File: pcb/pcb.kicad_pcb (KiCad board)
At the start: 2 copper layers, 152 x 91.6 mm, 66 parts, among them J1 USB_C_Receptacle_USB2.0_16P, J2 Conn_01x02, K1 SW_Push, K10 SW_Push, K11 SW_Push, K12 SW_Push, K13 SW_Push, K14 SW_Push, K15 SW_Push, K16 SW_Push, K17 SW_Push, K18 SW_Push, K19 SW_Push, K2 SW_Push, K20 SW_Push, K21 SW_Push, K3 SW_Push, K4 SW_Push, K5 SW_Push, K6 SW_Push, K7 SW_Push, K8 SW_Push, K9 SW_Push, U1 SRV05-4, U2 ProMicro, U3 SRV05-4

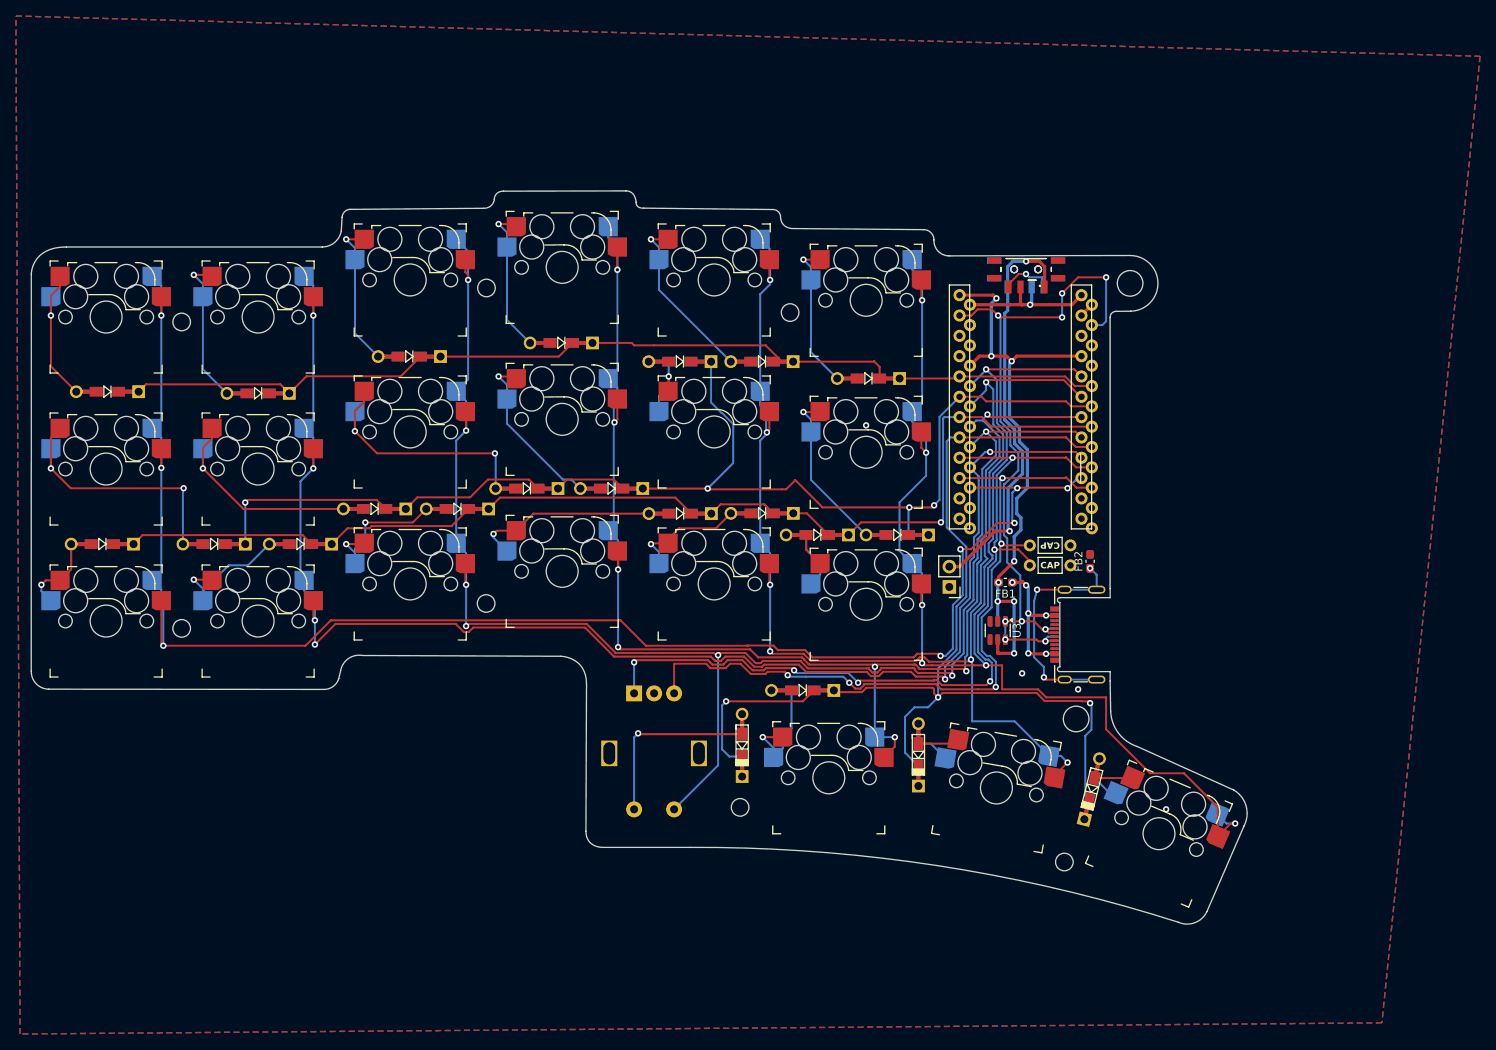
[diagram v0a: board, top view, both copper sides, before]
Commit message: cirrus40, second manufactured version
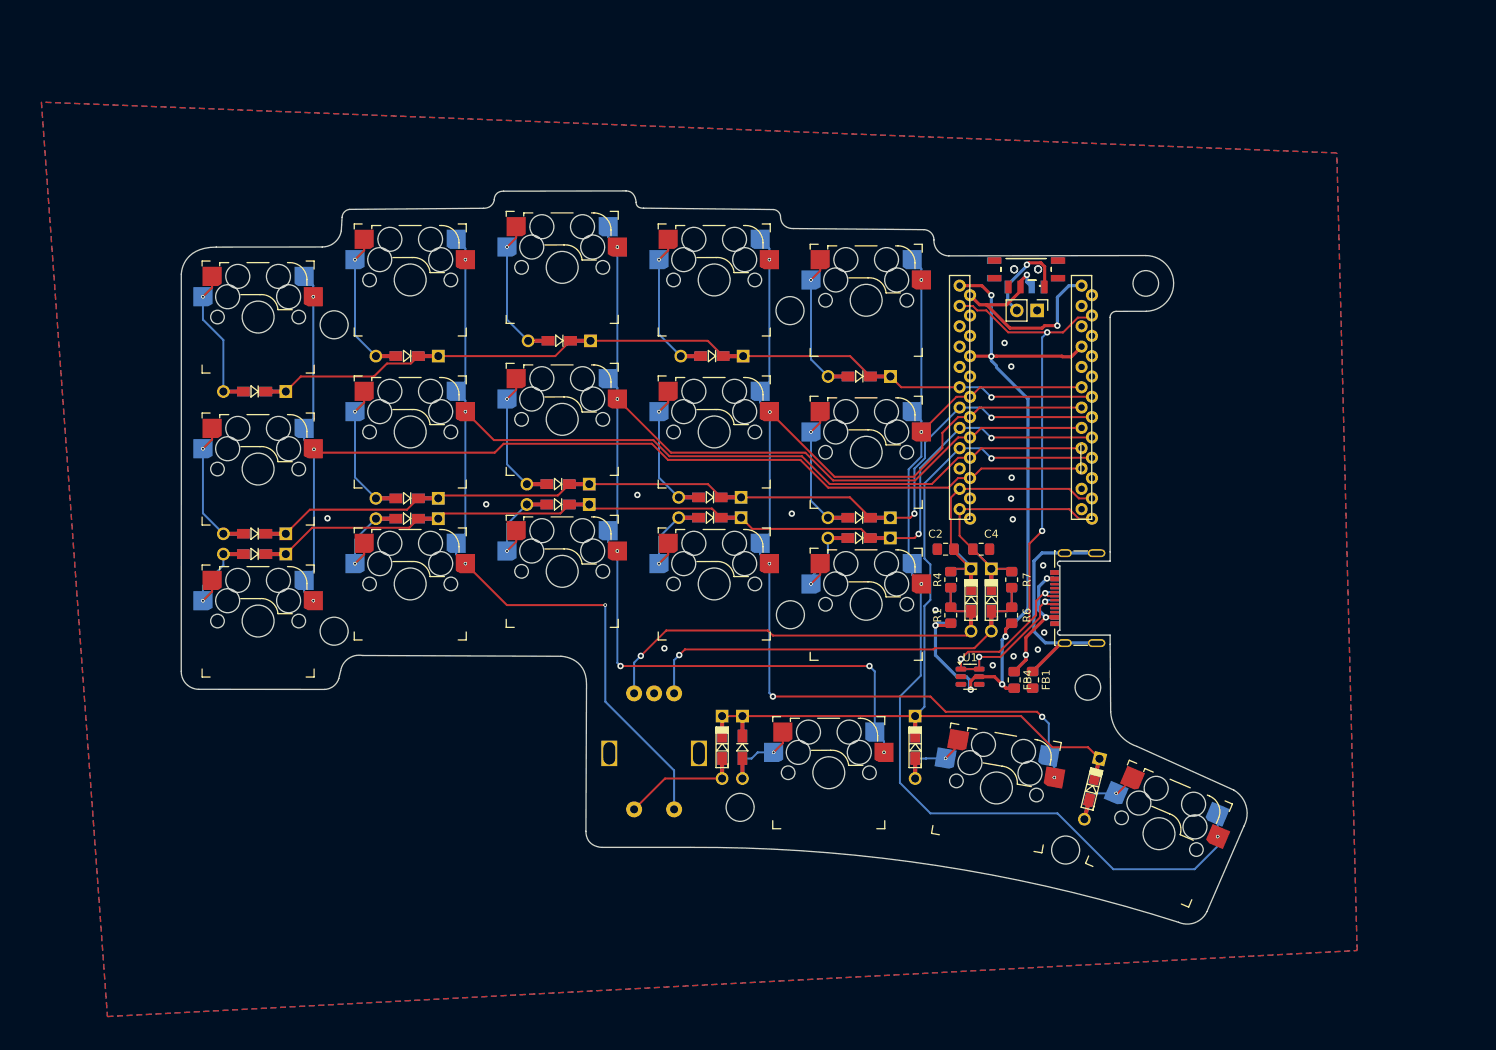
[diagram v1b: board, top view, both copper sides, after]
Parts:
- removed the D19 at (50.2, 74.3)
- removed the D20 at (63.5, 93.3)
- removed D22: DIODE, footprints:Diode-dual
- removed K19, K20, K21: SW_Push, footprints:SW_MX_HotSwap_Reversible
- removed the REF** at (97.5, 61.3)
- added C1: 470nF, Capacitor_SMD:C_0805_2012Metric_Pad1.18x1.45mm_HandSolder, B.Cu at (154.9, 94.0)
- added C3: 470nF, Capacitor_SMD:C_0805_2012Metric_Pad1.18x1.45mm_HandSolder, B.Cu at (159.4, 94.0)
- added D12: DIODE, footprints:Diode-dual, F.Cu at (158.1, 100.3)
- added D21: DIODE, footprints:Diode-dual, F.Cu at (160.7, 100.3)
- added R1: 10kOhm, Resistor_SMD:R_0805_2012Metric_Pad1.20x1.40mm_HandSolder, F.Cu at (155.6, 102.2)
- added R2: 10kOhm, Resistor_SMD:R_0805_2012Metric_Pad1.20x1.40mm_HandSolder, B.Cu at (155.6, 102.2)
- added R3: 8kOhm, Resistor_SMD:R_0805_2012Metric_Pad1.20x1.40mm_HandSolder, B.Cu at (155.6, 97.8)
- added R4: 8kOhm, Resistor_SMD:R_0805_2012Metric_Pad1.20x1.40mm_HandSolder, F.Cu at (155.6, 97.8)
- added R5: 10kOhm, Resistor_SMD:R_0805_2012Metric_Pad1.20x1.40mm_HandSolder, B.Cu at (163.2, 102.2)
- added R6: 10kOhm, Resistor_SMD:R_0805_2012Metric_Pad1.20x1.40mm_HandSolder, F.Cu at (163.2, 102.2)
- added R7: 8kOhm, Resistor_SMD:R_0805_2012Metric_Pad1.20x1.40mm_HandSolder, F.Cu at (163.2, 97.8)
- added R8: 8kOhm, Resistor_SMD:R_0805_2012Metric_Pad1.20x1.40mm_HandSolder, B.Cu at (163.2, 97.8)
- C2: renamed from C1; value 50V/100nF axial -> 470nF; footprint footprints:RESISTOR_Reversible -> Capacitor_SMD:C_0805_2012Metric_Pad1.18x1.45mm_HandSolder
- C4: renamed from C2; value 50V/100nF axial -> 470nF; footprint footprints:RESISTOR_Reversible -> Capacitor_SMD:C_0805_2012Metric_Pad1.18x1.45mm_HandSolder
- FB1: renamed from FB2; footprint footprints:C_0603_1608Metric_Pad1.08x0.95mm_HandSolder -> Capacitor_SMD:C_0805_2012Metric_Pad1.18x1.45mm_HandSolder
- FB2: renamed from FB3; footprint footprints:C_0603_1608Metric_Pad1.08x0.95mm_HandSolder -> Capacitor_SMD:C_0805_2012Metric_Pad1.18x1.45mm_HandSolder
- FB3: renamed from FB4; footprint footprints:C_0603_1608Metric_Pad1.08x0.95mm_HandSolder -> Capacitor_SMD:C_0805_2012Metric_Pad1.18x1.45mm_HandSolder
- FB4: renamed from FB1; footprint footprints:C_0603_1608Metric_Pad1.08x0.95mm_HandSolder -> Capacitor_SMD:C_0805_2012Metric_Pad1.18x1.45mm_HandSolder
- REF** (x6): value MountingHole_2.2mm_M2 -> MountingHole_3.5mm_TinyCourtyard; footprint MountingHole:MountingHole_2.2mm_M2 -> footprints:MountingHole_3.5mm_TinyCourtyard
- moved REF** 38.1 mm to (135.5, 102.2)
- moved J2 36.3 mm to (166.4, 64.1), turned to -90 degrees
- moved REF** 19.1 mm to (78.5, 65.9)
- moved REF** 19.1 mm to (78.5, 104.2)
- moved D14 17.4 mm to (125.5, 87.5)
- moved FB1 16.5 mm to (165.8, 110.3), turned to -90 degrees
- moved FB2 16.5 mm to (165.8, 110.3), turned to -90 degrees
- moved D2 15.3 mm to (68.6, 92.1)
- moved D10 15.3 mm to (106.5, 88.4)
- moved D5 15.0 mm to (87.6, 87.6)
- moved C2 13.2 mm to (154.9, 94.0), turned to 180 degrees
- moved FB3 12.2 mm to (163.5, 110.3), turned to -90 degrees
- moved FB4 12.2 mm to (163.5, 110.3), turned to -90 degrees
- moved D11 10.4 mm to (129.5, 118.7), turned to 90 degrees
- moved C4 8.63 mm to (159.4, 94.0), turned to 0 degrees
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- renumbered D13 to D1, D9 to D10, D18 to D11, D4 to D13, D5 to D14, D6 to D15, D17 to D16, D1 to D17, D2 to D18, D3 to D19, D14 to D2, D16 to D20, D15 to D3, D10 to D4, D11 to D5, D12 to D6, D21 to D7, D7 to D8, D8 to D9, K13 to K1, K18 to K10, K4 to K11, K5 to K12, K6 to K13, K17 to K14, K1 to K15, K2 to K16, K3 to K17, K16 to K18, K14 to K2, K15 to K3, K10 to K4, K11 to K5, K12 to K6, U3 to U1, U1 to U2, U2 to U3
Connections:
- C2 pad 1: ENCA -> ENCA_DB
- C4 pad 1: GND -> ENCB_DB
- C4 pad 2: ENCB -> GND
- U3 pad 2: ROW0 -> unconnected-(U3-GP2-Pad2)
- U3 pad 20: COL5 -> COL4
- U3 pad 22: COL4 -> COL3
- U3 pad 26: COL3 -> COL2
- U3 pad 27: COL2 -> COL1
- U3 pad 28: COL1 -> COL0
- U3 pad 29: COL0 -> unconnected-(U3-GP29-Pad29)
- U3 pad 3: ROW1 -> ROW0
- U3 pad 4: ROW2 -> ROW1
- U3 pad 5: ROW3 -> ROW2
- U3 pad 6: ENCA -> ROW3
- U3 pad 7: ENCB -> unconnected-(U3-GP7-Pad7)
- U3 pad 8: unconnected-(U2-GP8-Pad8)_1 -> ENCA_DB
- U3 pad 9: unconnected-(U2-GP9-Pad9) -> ENCB_DB
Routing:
- net COL5: track 202.3 -> 0.00 mm, vias 8 -> 0
- net ENCA: track 105.0 -> 58.5 mm, vias 6 -> 1
- net COL4: track 184.2 -> 142.7 mm, vias 6 -> 3
- net ENCB: track 95.8 -> 55.7 mm, vias 5 -> 1
- net /Batt: track 52.1 -> 12.2 mm, vias 2 -> 1
- net ROW1: track 143.1 -> 105.8 mm, vias 4 -> 2
- net ENCA_DB: track 0.00 -> 37.2 mm
- net COL0: track 176.6 -> 141.0 mm, vias 7 -> 4
- net ENCB_DB: track 0.00 -> 34.9 mm
- net Net-(D20-K) (its old number): track 32.6 -> 0.00 mm, vias 2 -> 0
- net ROW3: track 132.5 -> 102.9 mm, vias 3 -> 1
- net ROW2: track 127.8 -> 106.1 mm, vias 1 -> 2
- net ROW0: track 117.4 -> 96.4 mm, vias 0 -> 1
- net VCC: track 75.6 -> 96.4 mm, vias 8 -> 6
- net COL3: track 193.5 -> 174.3 mm, vias 7 -> 4
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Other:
- board size 152 x 91.6 mm -> 133.2 x 91.6 mm
